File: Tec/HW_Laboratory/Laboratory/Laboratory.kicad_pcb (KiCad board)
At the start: 2 copper layers, 100 x 100 mm, 13 parts, among them J2 Conn_01x08_Pin, J3 Conn_01x08_Pin, Q1 AO3401A, Q2 AO3401A, Q3 AO3401A, Q4 AO3401A, Q5 AO3401A, Q6 AO3401A, U1 74HC595, U2 INA3221

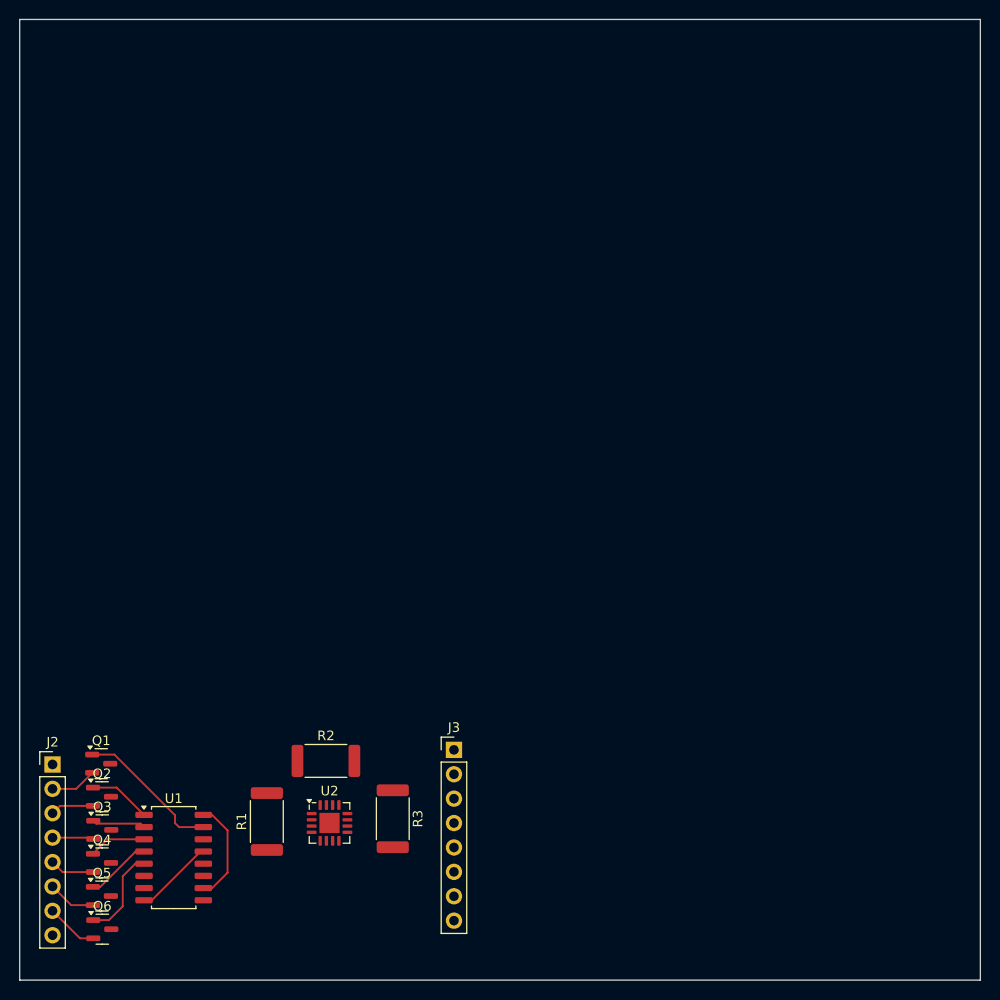
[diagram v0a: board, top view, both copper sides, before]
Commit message: New changes done
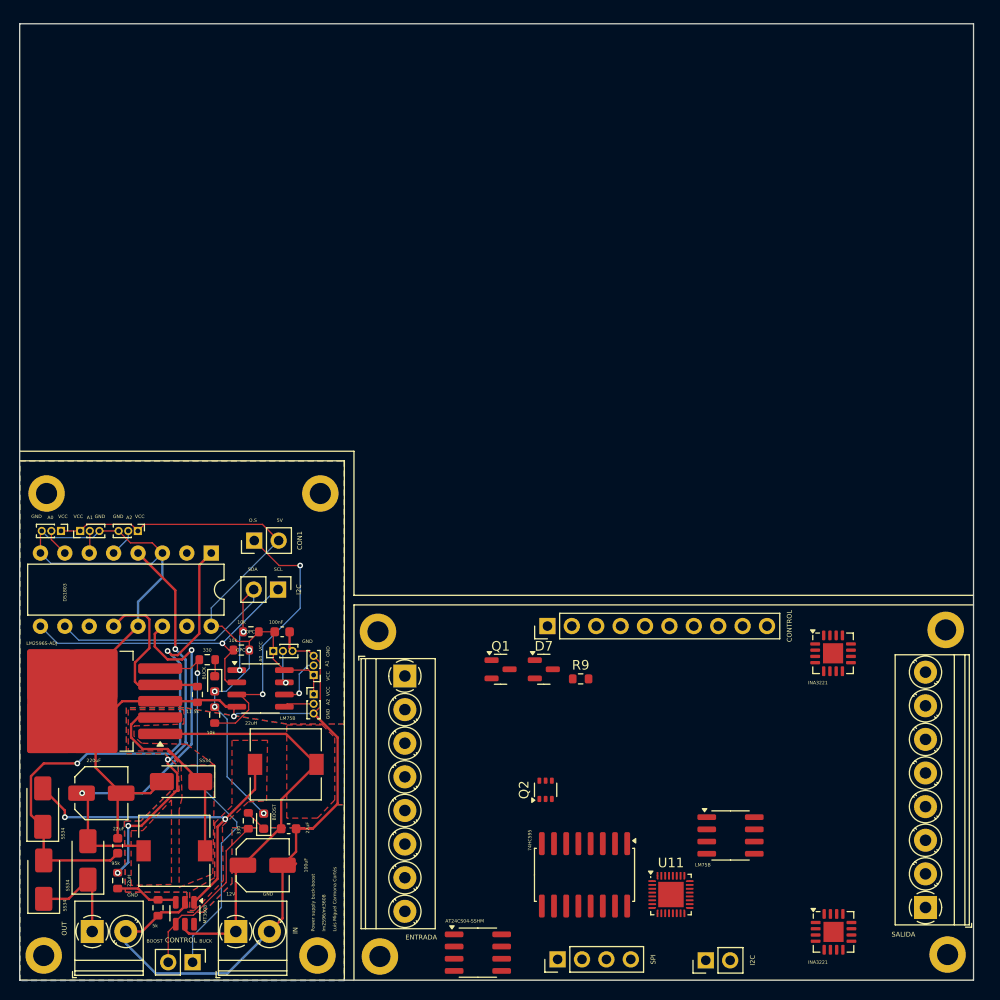
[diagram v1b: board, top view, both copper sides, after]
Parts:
- removed Q3, Q4, Q5, Q6: AO3401A, Package_TO_SOT_SMD:SOT-23
- added ?: , , F.Cu at (176.6, 103.6)
- added ?: , , F.Cu at (117.5, 103.8)
- added C1: 100uF, Capacitor_SMD:C_Elec_5x5.4, F.Cu at (105.5, 128.1)
- added C2: 220uF, Capacitor_SMD:C_Elec_5x5.4, F.Cu at (88.7, 120.6)
- added C3: 22uF, Capacitor_SMD:C_0603_1608Metric, F.Cu at (108.2, 124.3)
- added C4: 22uF, Capacitor_SMD:C_0603_1608Metric, F.Cu at (90.4, 126.1)
- added C5: 100nF, Capacitor_SMD:C_0603_1608Metric, F.Cu at (107.5, 103.8)
- added D1: SS34, Diode_SMD:D_SMA, F.Cu at (97.0, 119.4)
- added D2: SS34, Diode_SMD:D_SMA, F.Cu at (87.3, 127.6)
- added D3: SS34, Diode_SMD:D_SMA, F.Cu at (82.6, 122.1)
- added D4: SS34, Diode_SMD:D_SMA, F.Cu at (82.7, 129.6)
- added D5: BUCK, LED_SMD:LED_0603_1608Metric, F.Cu at (100.5, 109.2)
- added D6: BOOST, LED_SMD:LED_0603_1608Metric, F.Cu at (105.6, 123.5)
- added D7: BZX84Cxx, Package_TO_SOT_SMD:SOT-23, F.Cu at (134.8, 107.7)
- added H1: MountingHole_Pad, MountingHole:MountingHole_2.2mm_M2_DIN965_Pad, F.Cu at (83.0, 89.4)
- added H2: MountingHole_Pad, MountingHole:MountingHole_2.2mm_M2_DIN965_Pad, F.Cu at (111.5, 89.4)
- added H3: MountingHole_Pad, MountingHole:MountingHole_2.2mm_M2_DIN965_Pad, F.Cu at (82.7, 137.5)
- added H4: MountingHole_Pad, MountingHole:MountingHole_2.2mm_M2_DIN965_Pad, F.Cu at (111.2, 137.5)
- added J1: ENTRADA, TerminalBlock_Phoenix:TerminalBlock_Phoenix_PT-1,5-8-3.5-H_1x08_P3.50mm_Horizontal, F.Cu at (120.3, 108.4)
- added J10: SPI, Connector_PinHeader_2.54mm:PinHeader_1x04_P2.54mm_Vertical, F.Cu at (136.2, 137.9)
- added J11: A0, Connector_PinHeader_1.00mm:PinHeader_1x03_P1.00mm_Vertical, F.Cu at (84.5, 93.3)
- added J12: A1, Connector_PinHeader_1.00mm:PinHeader_1x03_P1.00mm_Vertical, F.Cu at (86.5, 93.3)
- added J13: I2C, Connector_PinHeader_2.54mm:PinHeader_1x02_P2.54mm_Vertical, F.Cu at (107.1, 99.4)
- added J14: CON1, Connector_PinHeader_2.54mm:PinHeader_1x02_P2.54mm_Vertical, F.Cu at (104.6, 94.3)
- added J15: I2C, Connector_PinHeader_2.54mm:PinHeader_1x02_P2.54mm_Vertical, F.Cu at (151.6, 138.0)
- added J16: CONTROL, Connector_PinHeader_2.54mm:PinHeader_1x10_P2.54mm_Vertical, F.Cu at (135.1, 103.2)
- added J4: CONTROL, Connector_PinHeader_2.54mm:PinHeader_1x02_P2.54mm_Vertical, F.Cu at (98.2, 138.2)
- added J5: OUT, TerminalBlock_Phoenix:TerminalBlock_Phoenix_PT-1,5-2-3.5-H_1x02_P3.50mm_Horizontal, F.Cu at (87.8, 135.0)
- added J6: A2, Connector_PinHeader_1.00mm:PinHeader_1x03_P1.00mm_Vertical, F.Cu at (92.5, 93.3)
- added J7: A0, Connector_PinHeader_1.00mm:PinHeader_1x03_P1.00mm_Vertical, F.Cu at (106.6, 105.8)
- added J8: A2, Connector_PinHeader_1.00mm:PinHeader_1x03_P1.00mm_Vertical, F.Cu at (110.8, 110.3)
- added J9: A1, Connector_PinHeader_1.00mm:PinHeader_1x03_P1.00mm_Vertical, F.Cu at (110.8, 108.3)
- added L1: 22uH, Inductor_SMD:L_7.3x7.3_H4.5, F.Cu at (96.3, 126.6)
- added L2: 22uH, Inductor_SMD:L_7.3x7.3_H4.5, F.Cu at (107.9, 117.6)
- added R4: 10k, Resistor_SMD:R_0603_1608Metric, F.Cu at (100.5, 112.5)
- added R5: 10k, Resistor_SMD:R_0603_1608Metric, F.Cu at (104.3, 103.8)
- added R6: 10k, Resistor_SMD:R_0603_1608Metric, F.Cu at (103.3, 105.7)
- added R7: 330, Resistor_SMD:R_0603_1608Metric, F.Cu at (99.7, 106.7)
- added R8: 330, Resistor_SMD:R_0603_1608Metric, F.Cu at (104.0, 123.5)
- added R9: 10k, Resistor_SMD:R_0603_1608Metric, F.Cu at (138.6, 108.7)
- added REF**: MountingHole_2.2mm_M2_DIN965_Pad, MountingHole:MountingHole_2.2mm_M2_DIN965_Pad, F.Cu at (176.8, 137.4)
- added REF**: MountingHole_2.2mm_M2_DIN965_Pad, MountingHole:MountingHole_2.2mm_M2_DIN965_Pad, F.Cu at (117.7, 137.6)
- added U10: LM75B, Package_SO:SOIC-8_3.9x4.9mm_P1.27mm, F.Cu at (105.3, 109.7)
- added U11: ch32v006k8u6, Package_DFN_QFN:QFN-32-1EP_4x4mm_P0.4mm_EP2.65x2.65mm, F.Cu at (148.0, 131.2)
- added U3: 74HC595, Package_SO:SOIC-16W_5.3x10.2mm_P1.27mm, F.Cu at (139.0, 129.1)
- added U5: INA3221, Package_DFN_QFN:Texas_RGV0016A_VQFN-16-1EP_4x4mm_P0.65mm_EP2.1x2.1mm, F.Cu at (164.9, 106.0)
- added U6: INA3221, Package_DFN_QFN:Texas_RGV0016A_VQFN-16-1EP_4x4mm_P0.65mm_EP2.1x2.1mm, F.Cu at (164.9, 135.0)
- added U7: LM75B, Package_SO:SOIC-8_3.9x4.9mm_P1.27mm, F.Cu at (154.2, 125.0)
- added U8: AT24CS04-SSHM, Package_SO:SOIC-8_3.9x4.9mm_P1.27mm, F.Cu at (127.9, 137.2)
- added U9: DS1803, Package_DIP:DIP-16_W7.62mm, F.Cu at (100.1, 95.6)
- J2: value Conn_01x08_Pin -> SALIDA; footprint Connector_PinHeader_2.54mm:PinHeader_1x08_P2.54mm_Vertical -> TerminalBlock_Phoenix:TerminalBlock_Phoenix_PT-1,5-8-3.5-H_1x08_P3.50mm_Horizontal
- J3: value Conn_01x08_Pin -> IN; footprint Connector_PinHeader_2.54mm:PinHeader_1x08_P2.54mm_Vertical -> TerminalBlock_Phoenix:TerminalBlock_Phoenix_PT-1,5-2-3.5-H_1x02_P3.50mm_Horizontal
- Q2: value AO3401A -> BC847BS; footprint Package_TO_SOT_SMD:SOT-23 -> Package_TO_SOT_SMD:SOT-363_SC-70-6
- R1: value 0.01 -> 11.5k; footprint Resistor_SMD:R_2512_6332Metric -> Resistor_SMD:R_0603_1608Metric
- R2: value 0.01 -> 5k; footprint Resistor_SMD:R_2512_6332Metric -> Resistor_SMD:R_0603_1608Metric
- R3: value 0.01 -> 95k; footprint Resistor_SMD:R_2512_6332Metric -> Resistor_SMD:R_0603_1608Metric
- U1: value 74HC595 -> LM2596S-ADJ; footprint Package_SO:SOP-16_4.4x10.4mm_P1.27mm -> Package_TO_SOT_SMD:TO-263-5_TabPin3
- U2: value INA3221 -> MT3608; footprint Package_DFN_QFN:Texas_RGV0016A_VQFN-16-1EP_4x4mm_P0.65mm_EP2.1x2.1mm -> Package_TO_SOT_SMD:SOT-23-6
- moved J2 92.1 mm to (174.5, 132.5), turned to 90 degrees
- moved Q2 46.2 mm to (134.9, 120.2), turned to 90 degrees
- moved Q1 42.7 mm to (130.3, 107.7)
- moved J3 29.6 mm to (102.7, 135.0)
- moved R3 29.4 mm to (90.4, 129.7)
- moved R2 23.2 mm to (94.6, 132.5), turned to 90 degrees
- moved U1 18.6 mm to (87.2, 111.0), turned to 180 degrees
- moved U2 17.7 mm to (97.4, 133.1), turned to -90 degrees
- moved R1 15.1 mm to (98.7, 110.3), turned to -90 degrees
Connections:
- J2 pad 1: /Fuente de alimentacion/Consumo/GND -> unconnected-(J2-Pin_1-Pad1)
- J2 pad 2: Net-(J2-Pin_2) -> unconnected-(J2-Pin_2-Pad2)
- J2 pad 3: Net-(J2-Pin_3) -> unconnected-(J2-Pin_3-Pad3)
- J2 pad 4: Net-(J2-Pin_4) -> unconnected-(J2-Pin_4-Pad4)
- J2 pad 5: Net-(J2-Pin_5) -> unconnected-(J2-Pin_5-Pad5)
- J2 pad 6: Net-(J2-Pin_6) -> unconnected-(J2-Pin_6-Pad6)
- J2 pad 7: Net-(J2-Pin_7) -> unconnected-(J2-Pin_7-Pad7)
- J2 pad 8: /Fuente de alimentacion/Consumo/GND -> unconnected-(J2-Pin_8-Pad8)
- J3 pad 1: /Fuente de alimentacion/Consumo/GND -> /Fuente_alimentacion/Regulador/Vin
- J3 pad 2: unconnected-(J3-Pin_2-Pad2) -> GND1
- Q1 pad 1: Net-(Q1-G) -> unconnected-(Q1-G-Pad1)
- Q1 pad 2: Net-(J2-Pin_2) -> unconnected-(Q1-S-Pad2)
- Q1 pad 3: /Fuente de alimentacion/Consumo/3.3V -> unconnected-(Q1-D-Pad3)
- Q2 pad 1: Net-(Q2-G) -> unconnected-(Q2A-E1-Pad1)
- Q2 pad 2: Net-(J2-Pin_3) -> unconnected-(Q2A-B1-Pad2)
- Q2 pad 3: /Fuente de alimentacion/Consumo/5V -> unconnected-(Q2B-C2-Pad3)
- R1 pad 1: Net-(J3-Pin_7) -> /Fuente_alimentacion/Regulador/FB_BUCK
- R1 pad 2: /Fuente de alimentacion/Consumo/3.3V -> GND1
- R2 pad 1: Net-(U2-IN+2) -> GND1
- R2 pad 2: /Fuente de alimentacion/Consumo/5V -> /Fuente_alimentacion/Regulador/FB_BOOST
- R3 pad 1: Net-(J3-Pin_5) -> Net-(U9-W1)
- R3 pad 2: /Fuente de alimentacion/Consumo/12V -> /Fuente_alimentacion/Regulador/FB_BOOST
- U1 pad 1: Net-(Q2-G) -> /Fuente_alimentacion/Regulador/Vin
- U1 pad 2: Net-(Q3-G) -> /Fuente_alimentacion/Regulador/OUT_BUCK
- U1 pad 3: Net-(Q4-G) -> GND1
- U1 pad 4: Net-(Q5-G) -> /Fuente_alimentacion/Regulador/FB_BUCK
- U1 pad 5: Net-(Q6-G) -> /Fuente_alimentacion/Regulador/BUCK
- U2 pad 1: /Fuente de alimentacion/Consumo/3.3V -> /Fuente_alimentacion/Regulador/SW_BOOST
- U2 pad 2: Net-(J3-Pin_7) -> GND1
- U2 pad 3: /Fuente de alimentacion/Consumo/GND -> /Fuente_alimentacion/Regulador/FB_BOOST
- U2 pad 4: unconnected-(U2-VS-Pad4) -> /Fuente_alimentacion/Regulador/BOOST
- U2 pad 5: /Fuente de alimentacion/Consumo/GND -> /Fuente_alimentacion/Regulador/Vin
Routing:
- net GND1: track 0.00 -> 155.6 mm, vias 0 -> 1
- net /Fuente_alimentacion/Regulador/5V: track 0.00 -> 75.7 mm, vias 0 -> 4
- net /Fuente_alimentacion/Regulador/Vout_boost: track 0.00 -> 57.8 mm, vias 0 -> 2
- net /Fuente_alimentacion/Regulador/Vin: track 0.00 -> 44.7 mm
- net /Fuente_alimentacion/Regulador/Vout_buck: track 0.00 -> 42.1 mm, vias 0 -> 2
- net Net-(U9-W1): track 0.00 -> 40.1 mm, vias 0 -> 4
- net /Fuente_alimentacion/Regulador/BUCK: track 0.00 -> 39.6 mm, vias 0 -> 1
- net /Fuente_alimentacion/Regulador/SW_BOOST: track 0.00 -> 37.9 mm, vias 0 -> 2
- net SCL: track 0.00 -> 34.0 mm, vias 0 -> 1
- net SDA: track 0.00 -> 32.2 mm, vias 0 -> 2
- net Net-(J14-Pin_1): track 0.00 -> 30.0 mm, vias 0 -> 2
- net /Fuente_alimentacion/Regulador/OUT_BUCK: track 0.00 -> 21.2 mm
- net /Fuente_alimentacion/Regulador/FB_BUCK: track 0.00 -> 18.2 mm
- net /Fuente_alimentacion/Regulador/BOOST: track 0.00 -> 18.1 mm
- net Net-(Q1-G): track 15.2 -> 0.00 mm
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- added copper zone on F.Cu, net /Fuente_alimentacion/Regulador/OUT_BUCK
- added copper zone on F.Cu, net /Fuente_alimentacion/Regulador/SW_BOOST
- added copper zone on F.Cu, net /Fuente_alimentacion/Regulador/Vin
- added copper zone on F.Cu, net /Fuente_alimentacion/Regulador/Vout_buck
- added copper zone on B.Cu, net GND1
- added copper zone on F.Cu, net GND1
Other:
- board size 100 x 100 mm -> 99.3 x 99.6 mm
- board text added: "12V"
- board text added: "5V"
- board text added: "BOOST"
- board text added: "BUCK"
- board text added: "GND"
- board text added: "O.S"
- board text added: "OPC"
- board text added: "Power supply buck-boost lm2596/mt3608 Luis Miguel Carmona Cortés"
- board text added: "SCL"
- board text added: "SDA"
- board text added: "VCC"
